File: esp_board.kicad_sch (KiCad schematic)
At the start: 4 parts, among them U1 ESP8285H16, U2 AP2205-33Y-13, U3 DS18B20

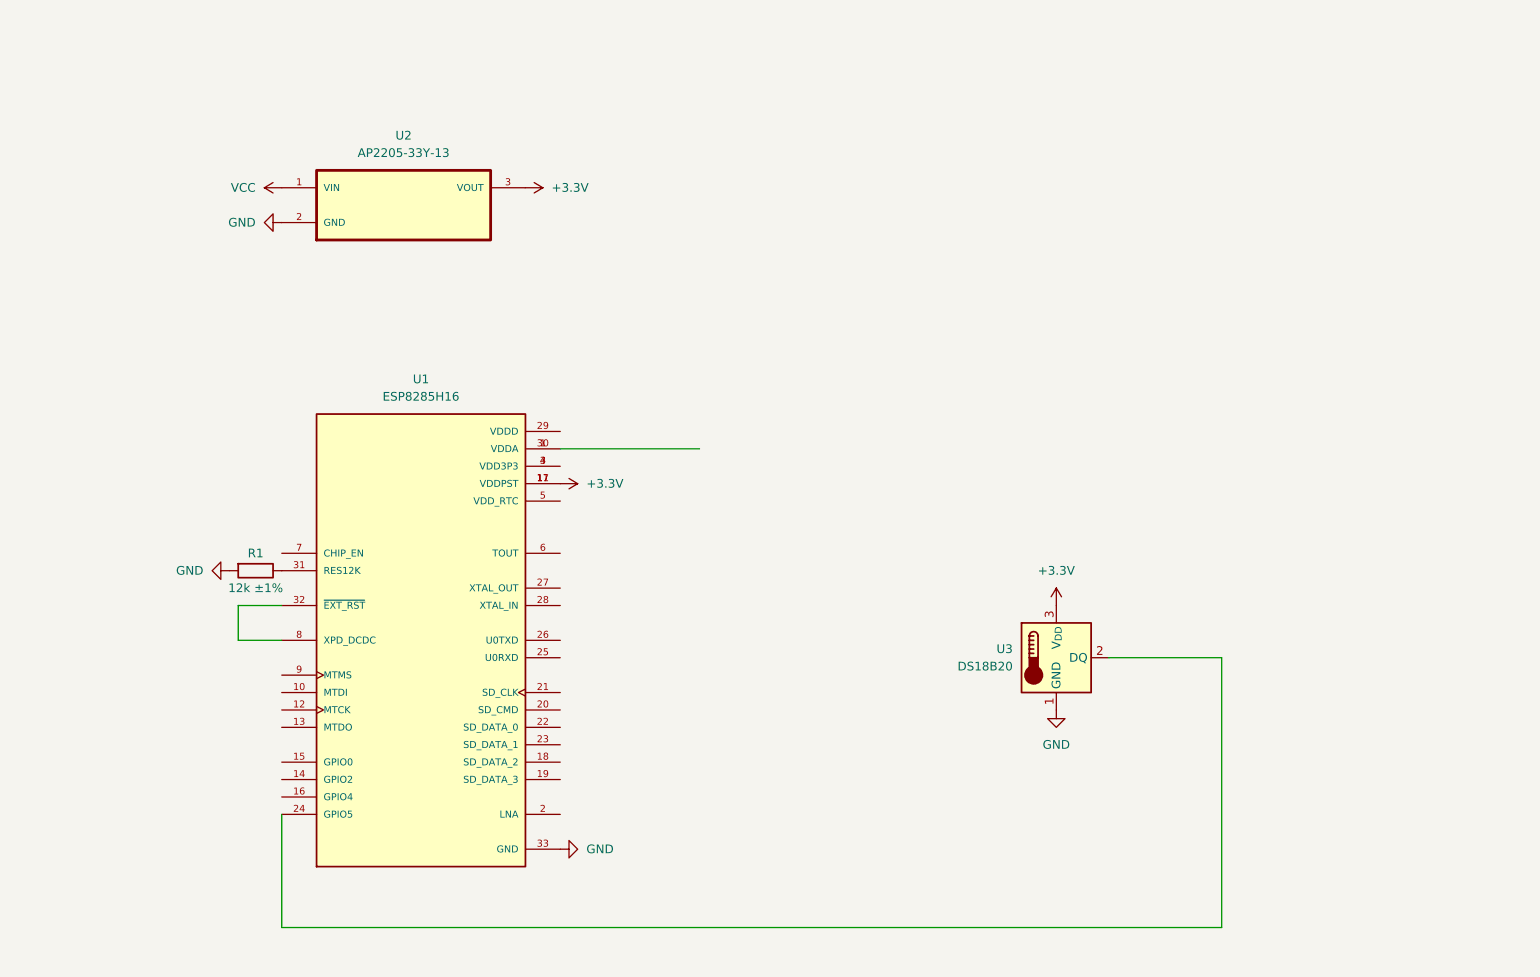
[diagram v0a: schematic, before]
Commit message: changed footprint, worked on power supply
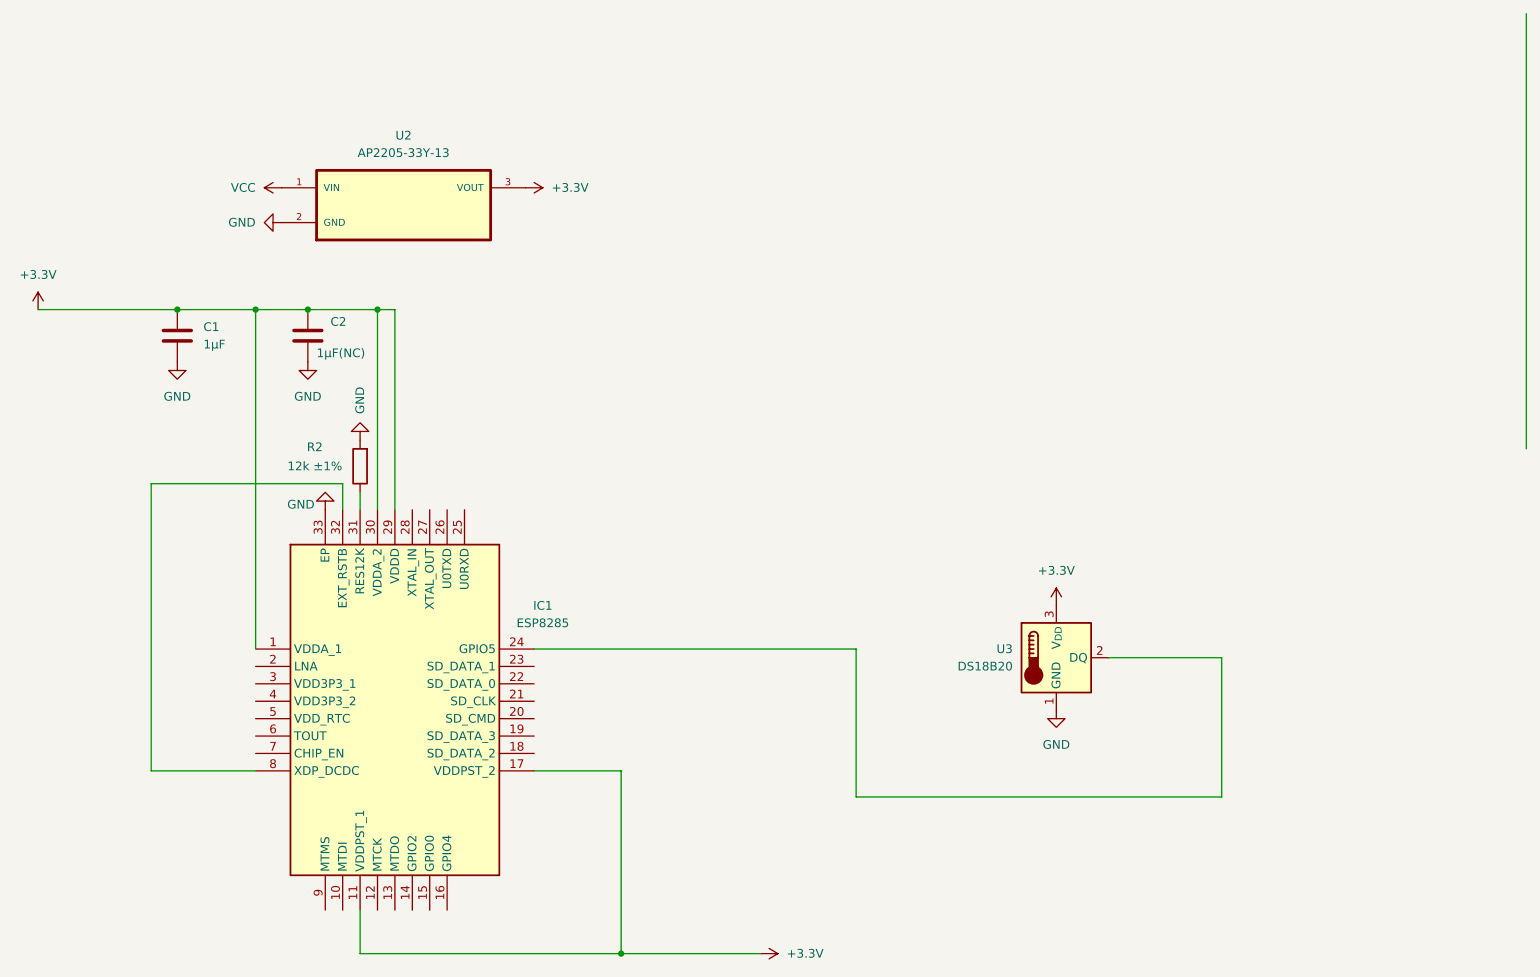
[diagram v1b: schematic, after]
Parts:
- removed R1: 12k ±1%, symbol Device:R
- removed U1: ESP8285H16, ESP8285H16:QFN50P500X500X90-33N, symbol custom:ESP8285H16
- added C1: 1μF, symbol Device:C
- added C2: 1μF(NC), symbol Device:C
- added IC1: ESP8285, QFN50P500X500X90-33N-D, symbol custom:ESP8285
- added R2: 12k ±1%, symbol Device:R
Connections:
- net +3.3V: now also C1.1, C2.1, IC1.1 (VDDA_1), IC1.11 (VDDPST_1), IC1.17 (VDDPST_2), IC1.29 (VDDD), IC1.30 (VDDA_2)
- net GND: now also C1.2, C2.2, IC1.33 (EP), R2.2
- net at U3.2 (DQ): now also IC1.24 (GPIO5)
- new net: IC1.31 (RES12K), R2.1
- new net: IC1.32 (EXT_RSTB), IC1.8 (XDP_DCDC)
